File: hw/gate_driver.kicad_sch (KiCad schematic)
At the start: 9 parts, among them U501 LMG1210RVRT

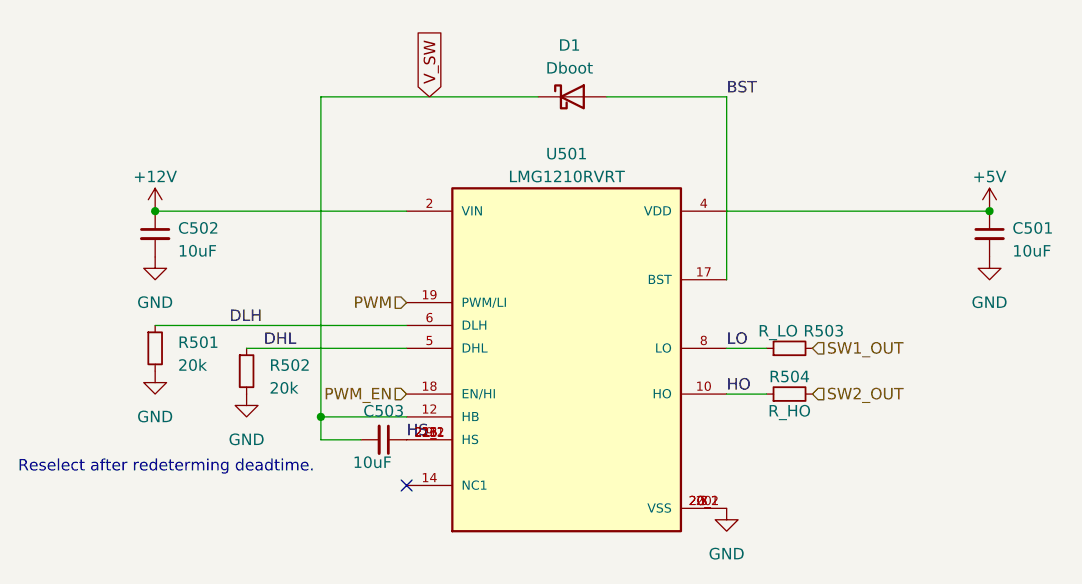
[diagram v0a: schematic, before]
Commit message: layout revision this one is cursed
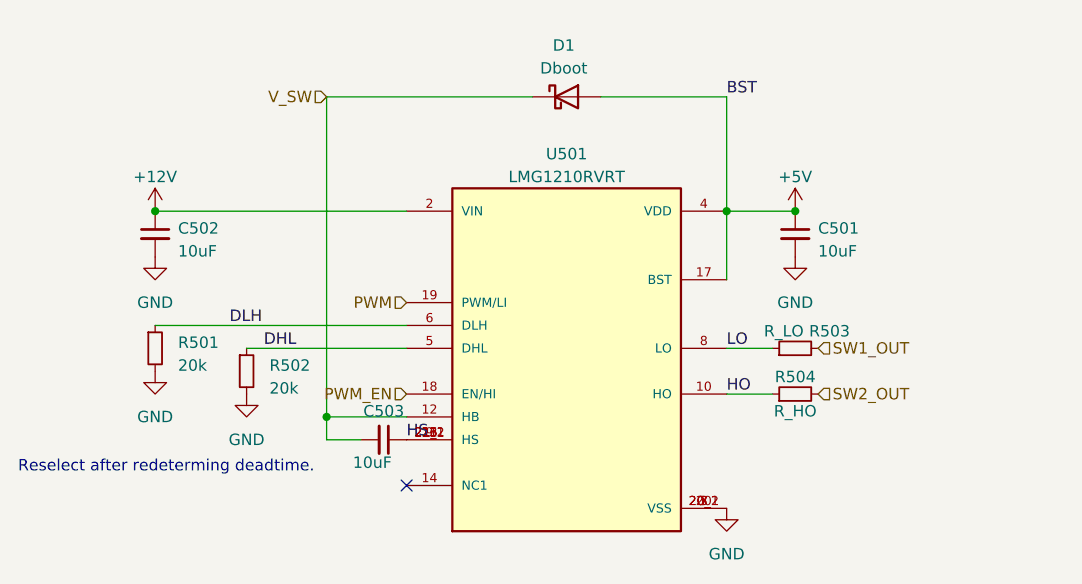
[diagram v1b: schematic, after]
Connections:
- net BST is gone; now on net +5V: D1.2 (A), U501.17 (BST)
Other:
- moved on the sheet: C501, D1, R503, R504

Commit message: slight bom updates
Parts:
- C501: In Stock? (none) -> Y; Mfg PN GRM158R61A226ME15D -> (none); Mfr PN (none) -> GRM158R61A226ME15D; Projected Cost (none) -> 0.48
- C502: In Stock? (none) -> Y; Projected Cost (none) -> 0.61
- C503: In Stock? (none) -> Y; Projected Cost (none) -> 0.48
- D1: In Stock? (none) -> Y; Projected Cost (none) -> 0.51
- U501: In Stock? (none) -> Y; Projected Cost (none) -> 4.10
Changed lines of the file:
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@@
       (effects (font (size 1.27 1.27)) hide)
     )
-    (property "Mfg PN" "GRM158R61A226ME15D" (at 181.61 81.28 0)
+    (property "Mfr PN" "GRM158R61A226ME15D" (at 181.61 81.28 0)
+      (effects (font (size 1.27 1.27)) hide)
+    )
+    (property "Projected Cost" "0.48" (at 181.61 81.28 0)
+      (effects (font (size 1.27 1.27)) hide)
+    )
+    (property "In Stock?" "Y" (at 181.61 81.28 0)
       (effects (font (size 1.27 1.27)) hide)
     )
@@
       (effects (font (size 1.27 1.27)) hide)
     )
+    (property "Projected Cost" "0.51" (at 156.21 66.04 0)
+      (effects (font (size 1.27 1.27)) hide)
+    )
+    (property "In Stock?" "Y" (at 156.21 66.04 0)
+      (effects (font (size 1.27 1.27)) hide)
+    )
     (pin "1")
     (pin "2")
@@
       (effects (font (size 1.27 1.27)) hide)
     )
+    (property "Projected Cost" "0.48" (at 135.89 104.14 90)
+      (effects (font (size 1.27 1.27)) hide)
+    )
+    (property "In Stock?" "Y" (at 135.89 104.14 90)
+      (effects (font (size 1.27 1.27)) hide)
+    )
     (pin "1")
     (pin "2")
@@
       (effects (font (size 1.27 1.27)) hide)
     )
+    (property "Projected Cost" "0.61" (at 110.49 81.28 0)
+      (effects (font (size 1.27 1.27)) hide)
+    )
+    (property "In Stock?" "Y" (at 110.49 81.28 0)
+      (effects (font (size 1.27 1.27)) hide)
+    )
     (pin "1")
     (pin "2")
@@
       (effects (font (size 1.27 1.27)) (justify bottom) hide)
     )
+    (property "Projected Cost" "4.10" (at 156.21 96.52 0)
+      (effects (font (size 1.27 1.27)) hide)
+    )
+    (property "In Stock?" "Y" (at 156.21 96.52 0)
+      (effects (font (size 1.27 1.27)) hide)
+    )
     (pin "10")
